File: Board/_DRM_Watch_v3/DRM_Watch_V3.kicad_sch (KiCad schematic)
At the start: 101 parts, among them J1 TYPE-C-31-M-12, J2 687110149022, Q1 2N7002LT1G, U1 ESP32-S2, U3 TP4056, U4 DS3231S, Y1 XRCGB48M000F0Z00R0

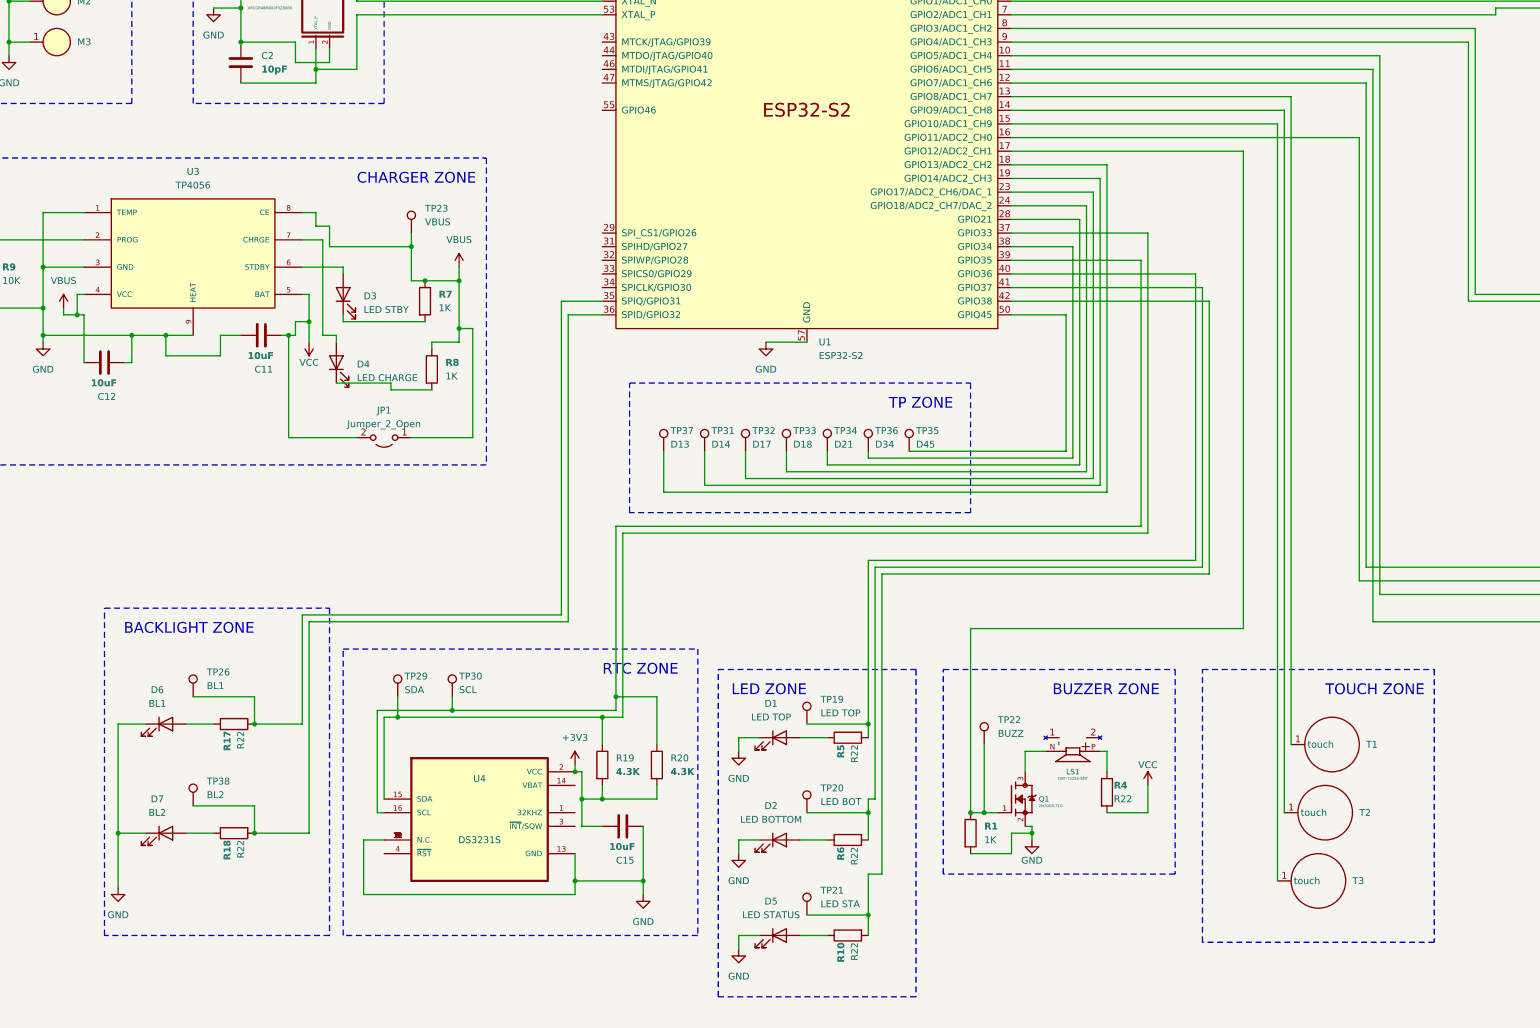
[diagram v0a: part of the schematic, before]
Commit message: bosrd
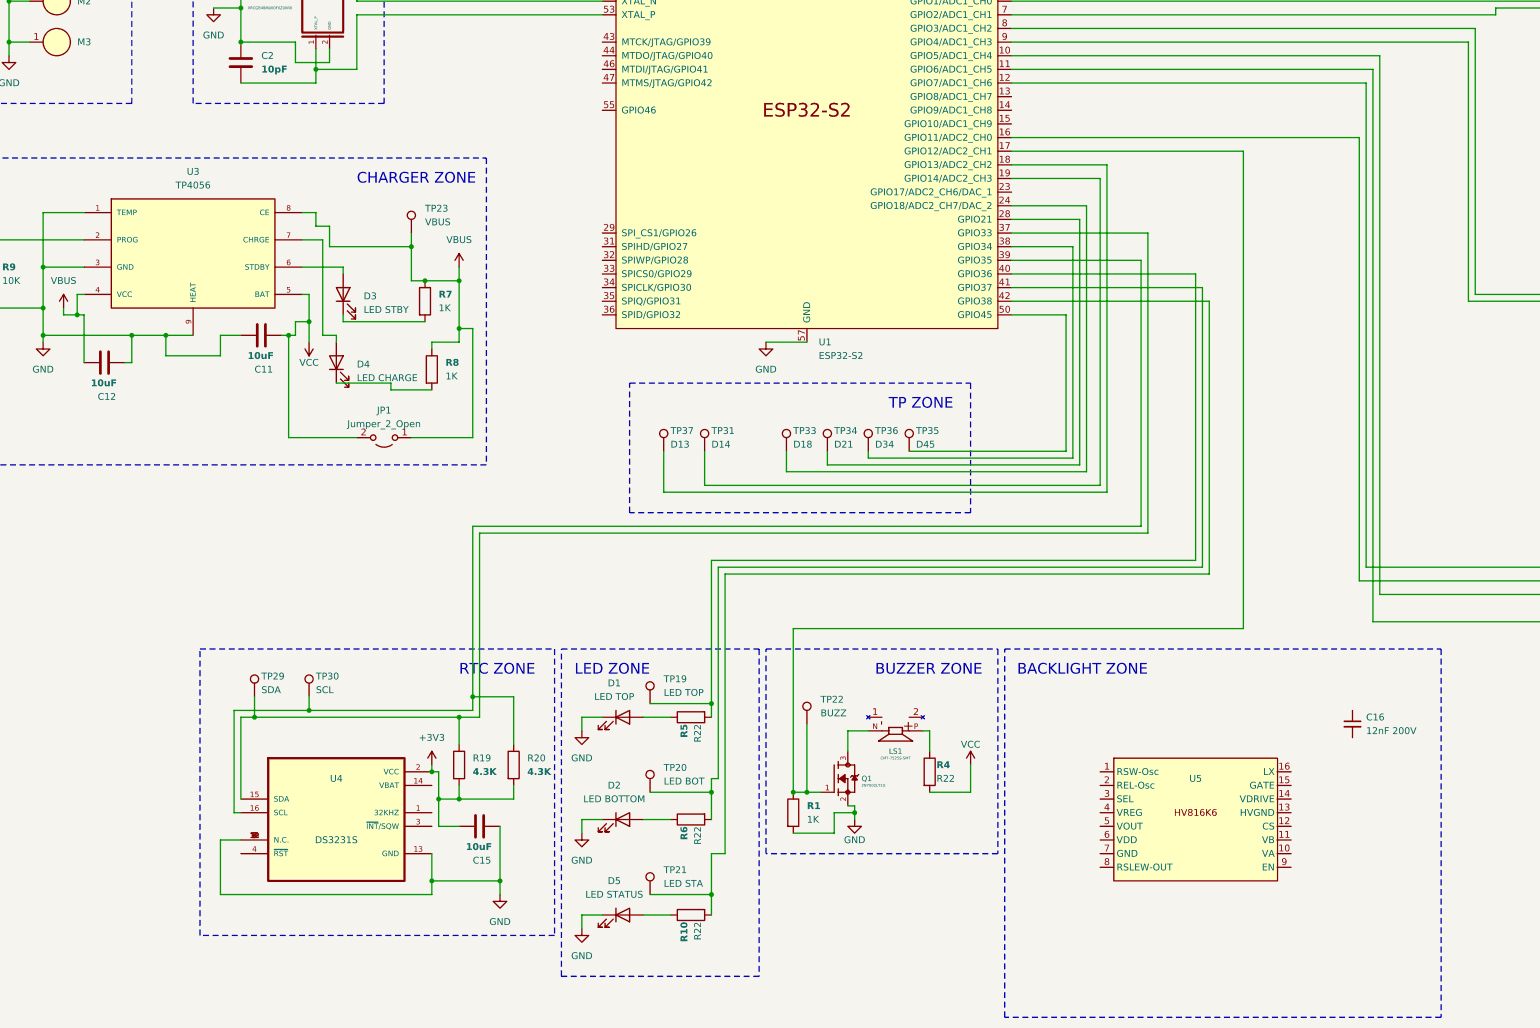
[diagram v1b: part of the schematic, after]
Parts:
- removed D6: BL1, Project-Lib:SMD-LED-Side-View, symbol Device:LED
- removed D7: BL2, Project-Lib:SMD-LED-Side-View, symbol Device:LED
- removed R17, R18: R22, Project-Lib:R_0603_1608Metric, symbol Device:R
- removed T1, T2, T3: ~, Project-Lib:Touch-Region, symbol Project-Lib:touch-region
- removed TP26: BL1, Project-Lib:TestPoint_Pad, symbol Project-Lib:TestPoint
- removed TP32: D17, Project-Lib:TestPoint_Pad, symbol Project-Lib:TestPoint
- removed TP38: BL2, Project-Lib:TestPoint_Pad, symbol Project-Lib:TestPoint
- added C16: 12nF 200V, Capacitor_SMD:C_1206_3216Metric, symbol Device:C_Small
- added U5: ~, Package_DFN_QFN:QFN-16-1EP_4x4mm_P0.65mm_EP2.5x2.5mm, symbol Project-Lib:HV816K6
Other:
- note removed: "TOUCH ZONE"
- moved on the sheet: C15, D1, D2, D5, LS1, Q1, R1, R10, R19, R20, R4, R5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
